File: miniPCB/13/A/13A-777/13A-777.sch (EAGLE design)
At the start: 92 parts, among them Q1 JFET-N, SOT23, Q2 JFET-N, SOT23, Q3 JFET-N, SOT23, Q4 JFET-N, SOT23, Q5 NTR2101P, Q6 NTR2101P, SW1 PEL12T, U2 MCP4451-502E/ML

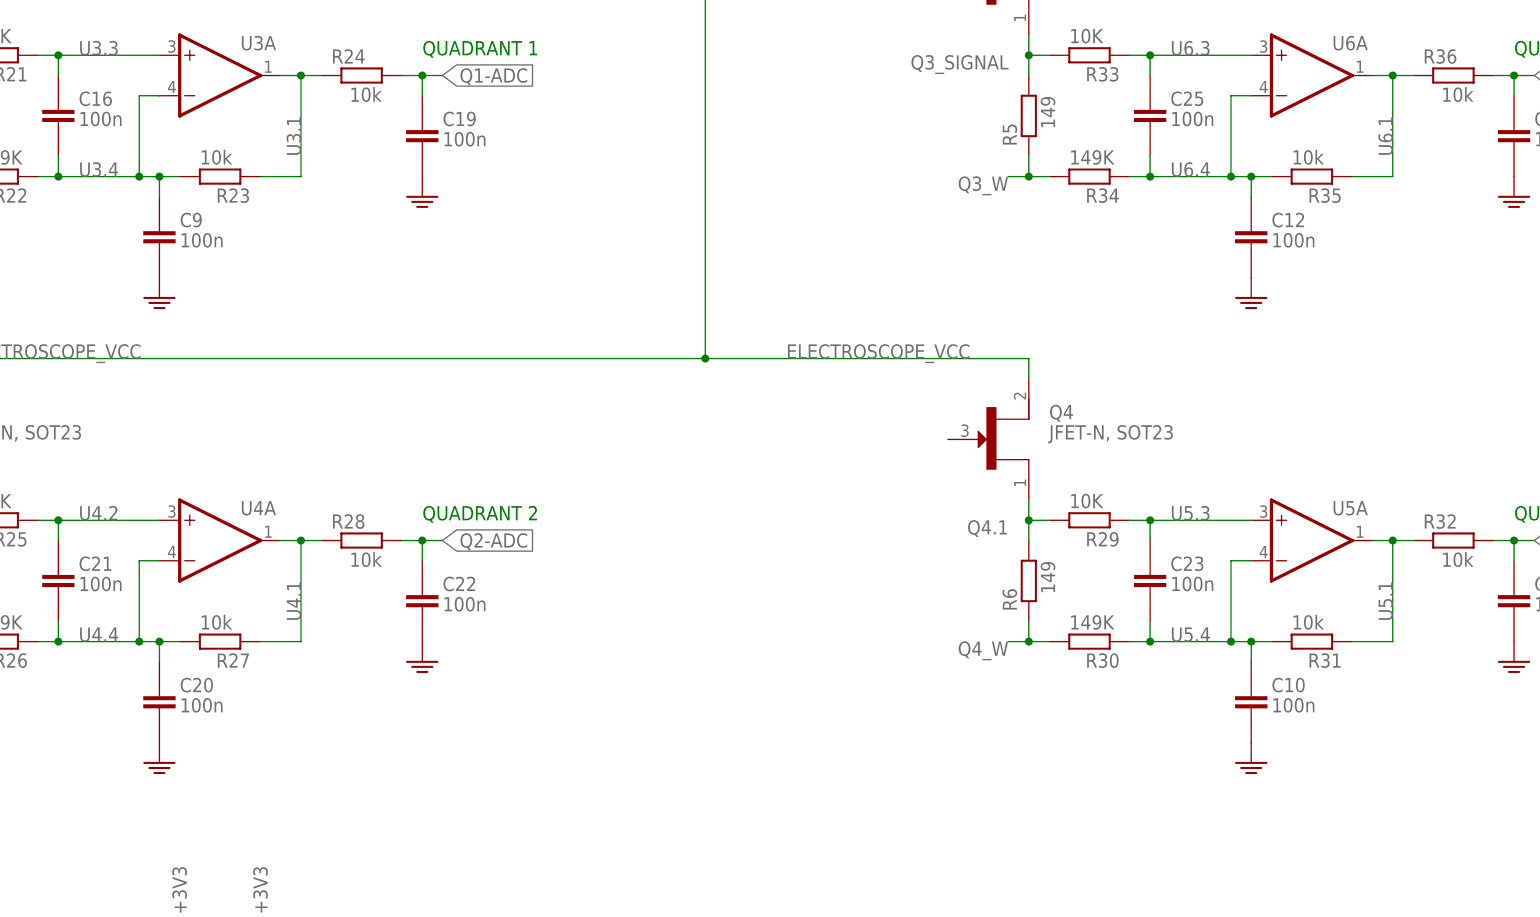
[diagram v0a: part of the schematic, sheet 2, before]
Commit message: NM.17JAN2023
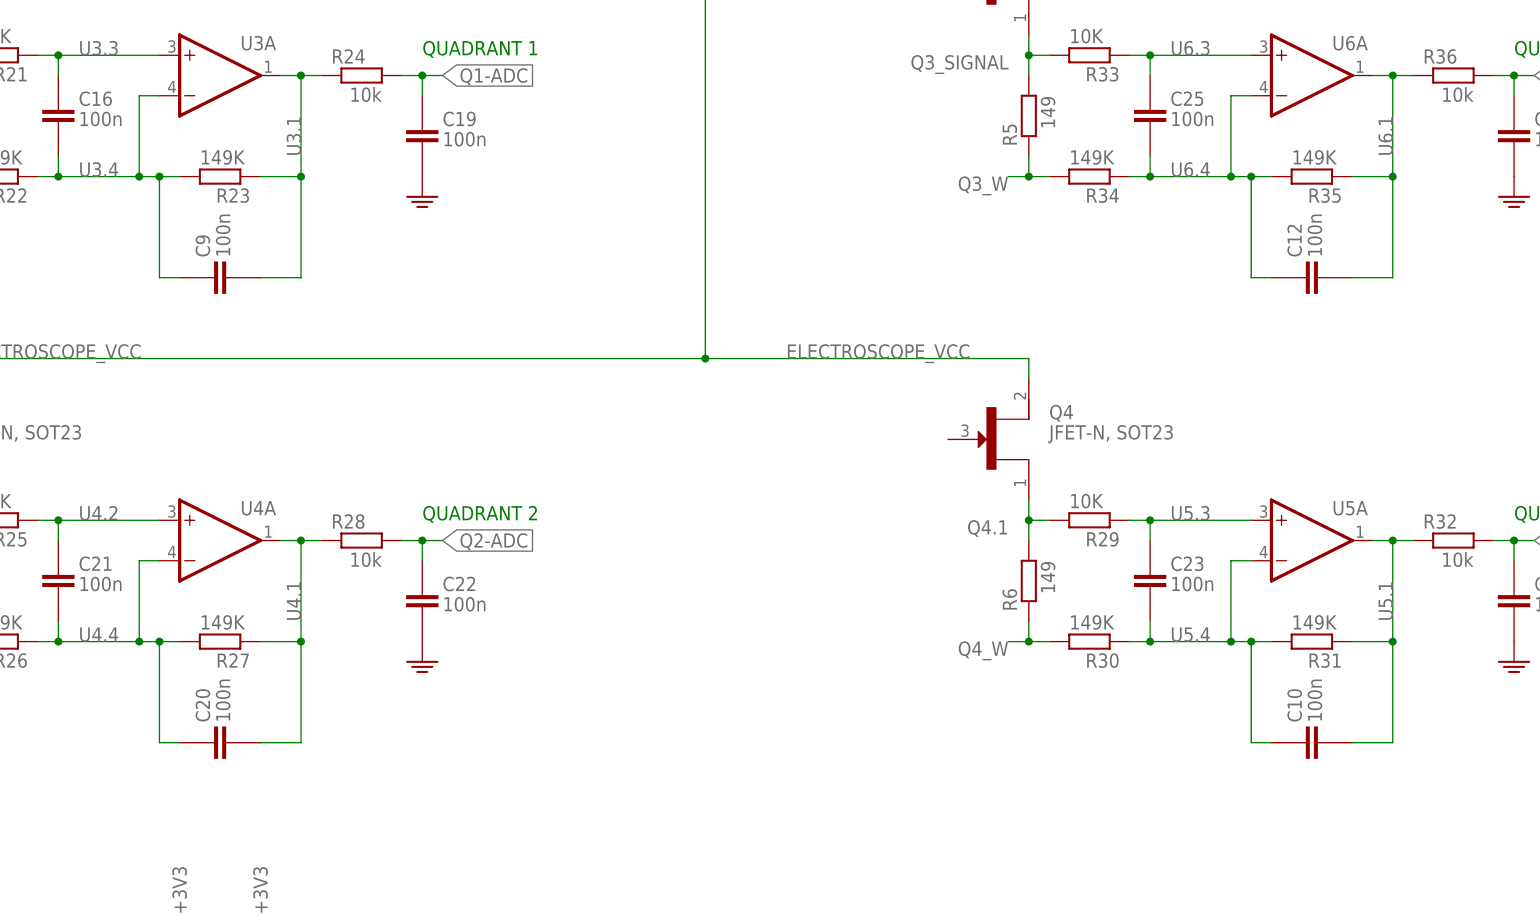
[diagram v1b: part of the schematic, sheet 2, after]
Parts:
- R23, R27, R31, R35: value 10k -> 149K
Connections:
- net GND: no longer C10.-, C12.-, C20.-, C9.-
- net U3.1: now also C9.-
- net U4.1: now also C20.-
- net U5.1: now also C10.-
- net U6.1: now also C12.-
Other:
- moved on the sheet: C10, C12, C20, C9
